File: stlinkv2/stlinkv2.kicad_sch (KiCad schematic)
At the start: 86 parts, among them J1 STLSWD, J2 JTAG, J3 SWD, J4 CLONE, J5 DBG_UART, J6 STM8, J7 POWER, J8 POWER, J9 USB_B_Mini, SW1 EXRERNAL POWER, U1 STM32F103CBTx, U2 74LVCC3245, U3 LD3985M33R_SOT23, U4 USBLC6-2, U5 ADUM3160, Y1 8MHz

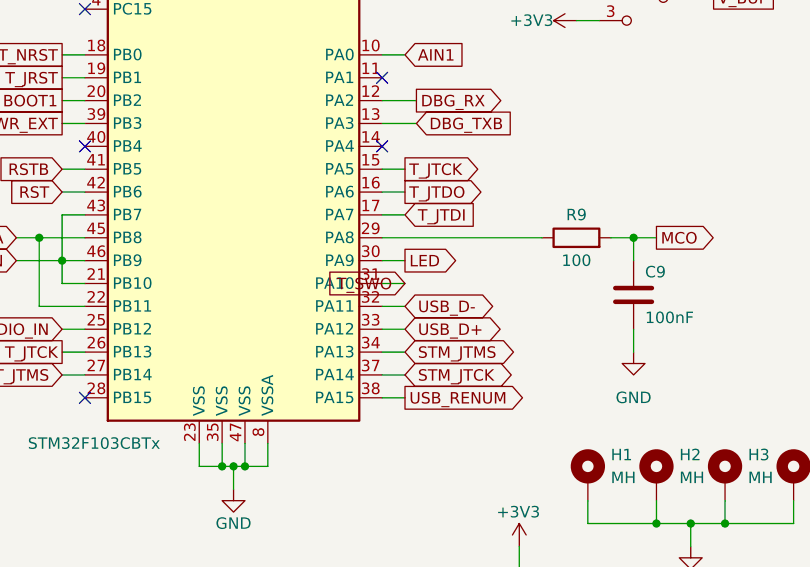
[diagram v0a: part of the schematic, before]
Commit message: update schema and pcb
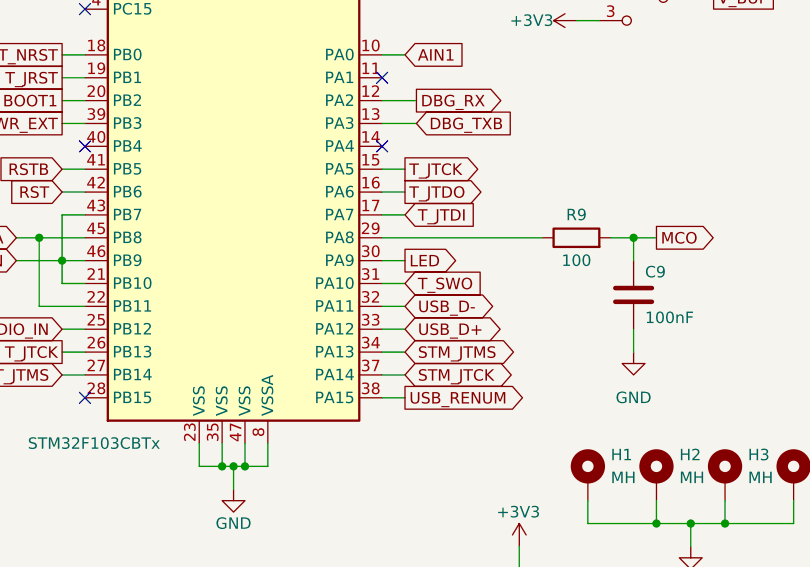
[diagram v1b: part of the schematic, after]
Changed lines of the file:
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@@
     )
   )
-  (global_label "T_SWO" (shape input) (at 132.08 86.36 180) (fields_autoplaced)
-    (effects (font (size 1.27 1.27)) (justify right))
-    (property "Intersheet References" "${INTERSHEET_REFS}" (id 0) (at 123.7402 86.2806 0)
-      (effects (font (size 1.27 1.27)) (justify right) hide)
+  (global_label "T_SWO" (shape input) (at 132.08 86.36 0) (fields_autoplaced)
+    (effects (font (size 1.27 1.27)) (justify left))
+    (property "Intersheet References" "${INTERSHEET_REFS}" (id 0) (at 140.4198 86.2806 0)
+      (effects (font (size 1.27 1.27)) (justify left) hide)
     )
   )
